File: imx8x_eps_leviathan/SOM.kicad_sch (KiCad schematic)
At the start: 3 parts, among them J10 BTH-070-02-L-D-A, J9 BTH-070-02-L-D-A (A to B)

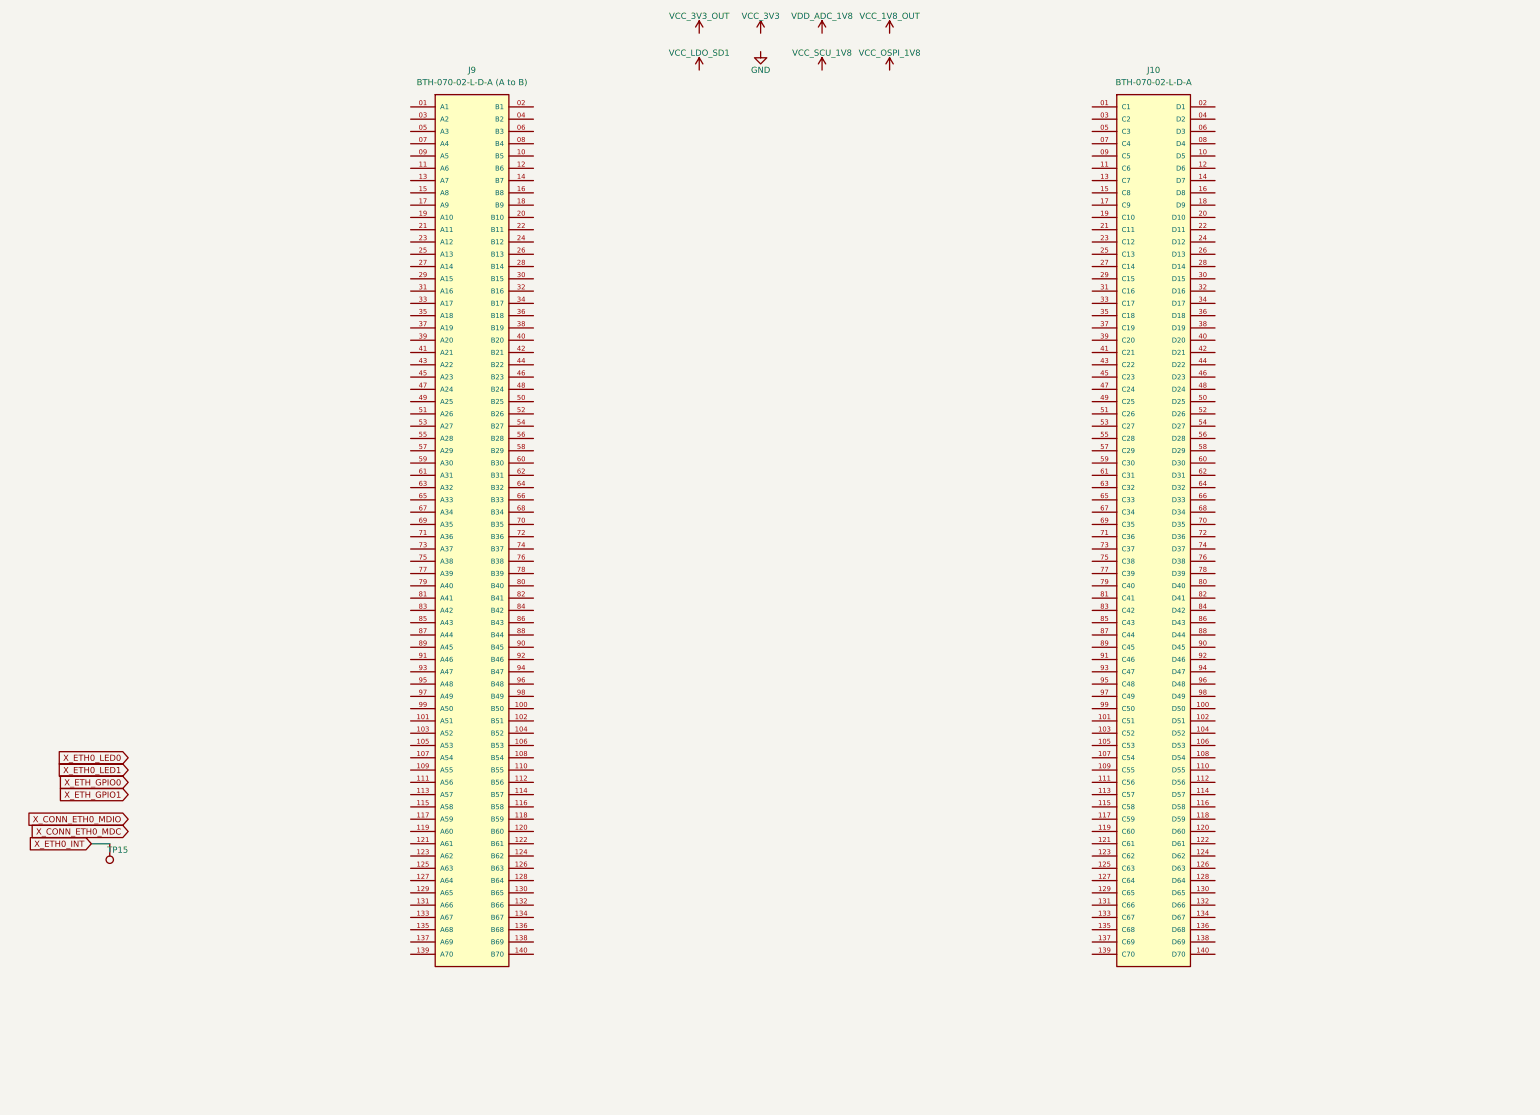
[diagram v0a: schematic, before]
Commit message: good stufff
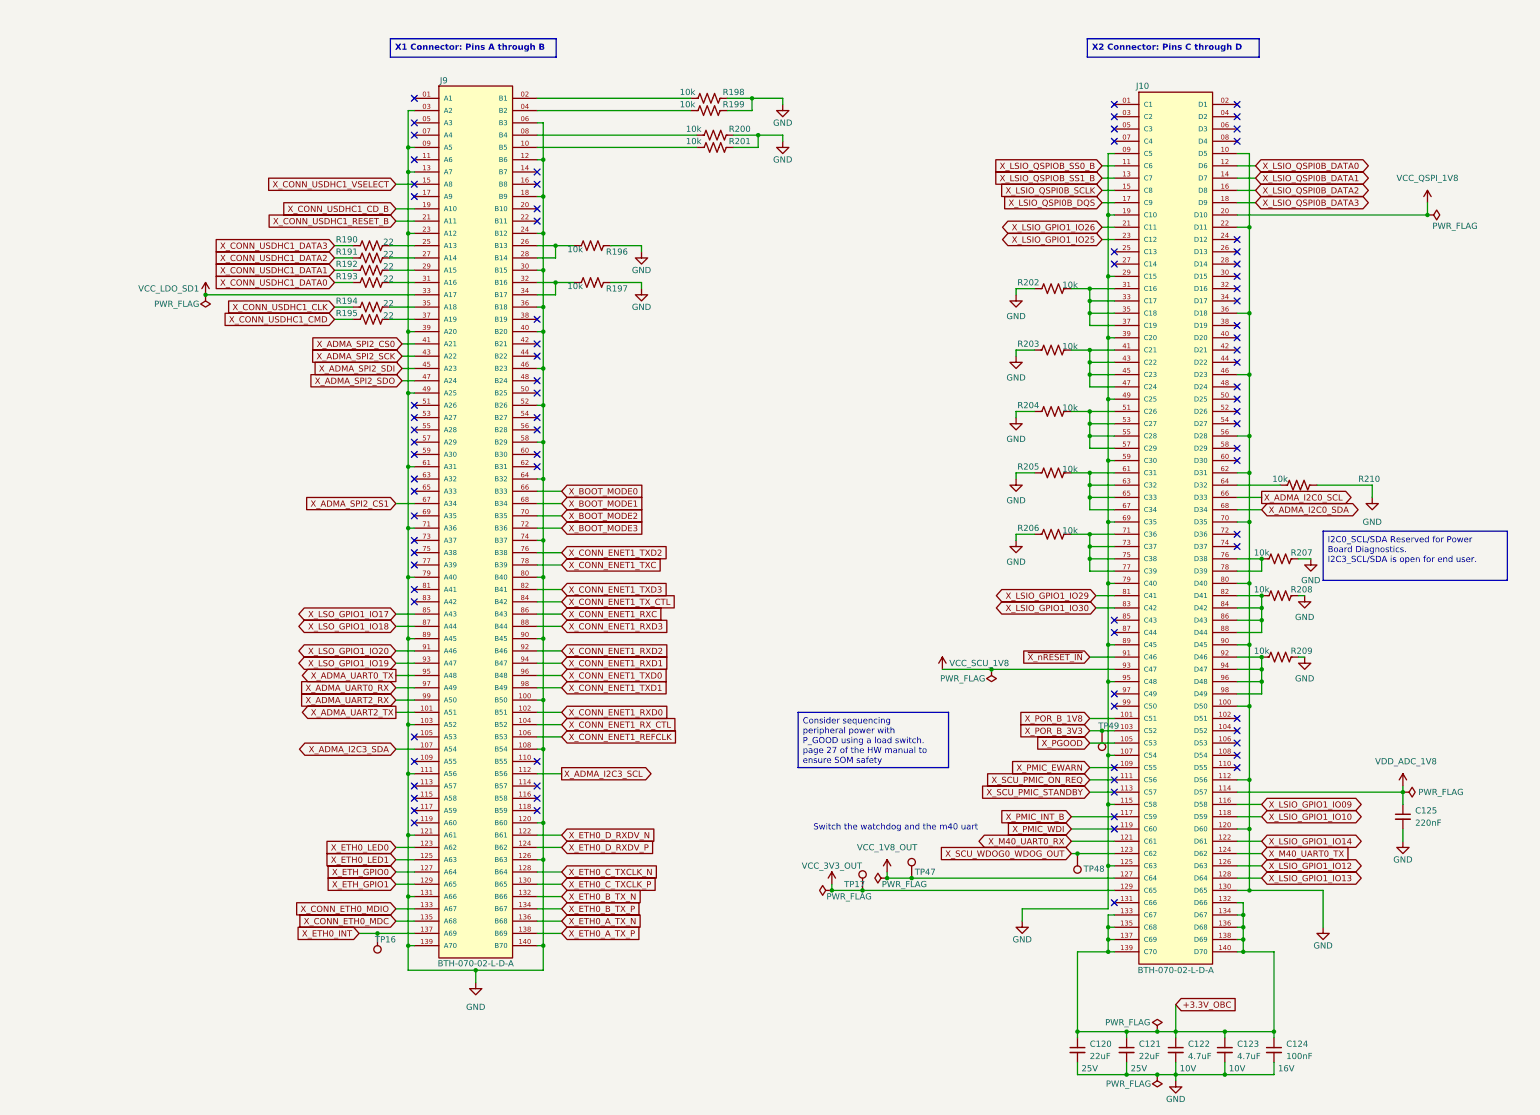
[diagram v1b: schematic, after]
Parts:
- removed TP15: TestPoint, TestPoint:TestPoint_THTPad_1.0x1.0mm_Drill0.5mm, symbol Connector:TestPoint
- added C120, C121: 22uF, Capacitor_SMD:C_0603_1608Metric, symbol Device:C_Small
- added C122, C123: 4.7uF, Capacitor_SMD:C_0603_1608Metric, symbol Device:C_Small
- added C124: 100nF, Capacitor_SMD:C_0603_1608Metric, symbol Device:C_Small
- added C125: 220nF, Capacitor_SMD:C_0603_1608Metric, symbol Device:C_Small
- added R190, R191, R192, R193, R194, R195: 22, Resistor_SMD:R_0402_1005Metric, symbol Device:R_US
- added R196, R197, R198, R199, R200, R201, R202, R203, R204, R205, R206, R207, R208, R209, R210: 10k, Resistor_SMD:R_0402_1005Metric, symbol Device:R_US
- added TP16, TP17, TP47, TP48, TP49: TestPoint, TestPoint:TestPoint_THTPad_1.0x1.0mm_Drill0.5mm, symbol Connector:TestPoint
- J9: value BTH-070-02-L-D-A (A to B) -> BTH-070-02-L-D-A
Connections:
- net GND: now also J10.09 (C5), J10.10 (D5), J10.100 (D50), J10.107 (C54), J10.112 (D56), J10.115 (C58), J10.120 (D60), J10.125 (C63), J10.130 (D65), J10.19 (C10), J10.22 (D11), J10.29 (C15), J10.36 (D18), J10.39 (C20), J10.46 (D23), J10.49 (C25), J10.56 (D28), J10.59 (C30), J10.62 (D31), J10.69 (C35), J10.70 (D35), J10.79 (C40), J10.80 (D40), J10.89 (C45), J10.90 (D45), J10.95 (C48), J9.03 (A2), J9.06 (B3), J9.09 (A5), J9.100 (B50), J9.103 (A52), J9.108 (B54), J9.111 (A56), J9.12 (B6), J9.120 (B60), J9.121 (A61), J9.126 (B63), J9.13 (A7), J9.131 (A66), J9.139 (A70), J9.140 (B70), J9.18 (B9), J9.23 (A12), J9.24 (B12), J9.30 (B15), J9.36 (B18), J9.39 (A20), J9.40 (B20), J9.46 (B23), J9.49 (A25), J9.52 (B26), J9.58 (B29), J9.61 (A31), J9.64 (B32), J9.71 (A36), J9.74 (B37), J9.79 (A40), J9.80 (B40), J9.89 (A45), J9.90 (B45), C120.2, C121.2, C122.2, C123.2, C124.2, C125.2, R196.1, R197.1, R198.1, R199.1, R200.1, R201.1, R202.1, R203.1, R204.1, R205.1, R206.1, R207.1, R208.1, R209.1, R210.1
- net VCC_1V8_OUT: now also J10.127 (C64), TP47.1
- net VCC_3V3_OUT: now also J10.129 (C65), TP17.1
- net VCC_LDO_SD1: now also J9.33 (A17)
- net VCC_SCU_1V8: now also J10.93 (C47)
- net VDD_ADC_1V8: now also J10.114 (D57), C125.1
- net X_CONN_ETH0_MDC: now also J9.135 (A68)
- net X_CONN_ETH0_MDIO: now also J9.133 (A67)
- net X_ETH0_INT: now also J9.137 (A69), TP16.1
- net X_ETH0_LED0: now also J9.123 (A62)
- net X_ETH0_LED1: now also J9.125 (A63)
- net X_ETH_GPIO0: now also J9.127 (A64)
- net X_ETH_GPIO1: now also J9.129 (A65)
- net X_POR_B_1V8: now reaches J10.101 (C51)
- net X_POR_B_3V3: now reaches J10.103 (C52)
- net X_POR_B_3V3: now also TP49.1
- net X_PGOOD: now reaches J10.105 (C53)
- net X_PMIC_EWARN: now reaches J10.109 (C55)
- net X_LSIO_QSPIOB_SS0_B: now reaches J10.11 (C6)
- net X_SCU_PMIC_ON_REQ: now reaches J10.111 (C56)
- net X_SCU_PMIC_STANDBY: now reaches J10.113 (C57)
- net X_LSIO_GPIO1_IO09: now reaches J10.116 (D58)
- net X_PMIC_INT_B: now reaches J10.117 (C59)
- net X_LSIO_GPIO1_IO10: now reaches J10.118 (D59)
- net X_PMIC_WDI: now reaches J10.119 (C60)
- net X_LSIO_QSPI0B_DATA0: now reaches J10.12 (D6)
- net X_M40_UART0_RX: now reaches J10.121 (C61)
- net X_LSIO_GPIO1_IO14: now reaches J10.122 (D61)
- net X_SCU_WDOG0_WDOG_OUT: now reaches J10.123 (C62)
- net X_SCU_WDOG0_WDOG_OUT: now also TP48.1
- net X_M40_UART0_TX: now reaches J10.124 (D62)
- net X_LSIO_GPIO1_IO12: now reaches J10.126 (D63)
- net X_LSIO_GPIO1_IO13: now reaches J10.128 (D64)
- net X_LSIO_QSPIOB_SS1_B: now reaches J10.13 (C7)
- net +3.3V_OBC: now reaches J10.132 (D66)
- net +3.3V_OBC: now also J10.133 (C67), J10.134 (D67), J10.135 (C68), J10.136 (D68), J10.137 (C69), J10.138 (D69), J10.139 (C70), J10.140 (D70), C120.1, C121.1, C122.1, C123.1, C124.1
- net X_LSIO_QSPI0B_DATA1: now reaches J10.14 (D7)
- net X_LSIO_QSPI0B_SCLK: now reaches J10.15 (C8)
- net X_LSIO_QSPI0B_DATA2: now reaches J10.16 (D8)
- net X_LSIO_QSPI0B_DQS: now reaches J10.17 (C9)
- net X_LSIO_QSPI0B_DATA3: now reaches J10.18 (D9)
- net VCC_QSPI_1V8: now reaches J10.20 (D10)
- net X_LSIO_GPIO1_IO26: now reaches J10.21 (C11)
- net X_LSIO_GPIO1_IO25: now reaches J10.23 (C12)
- net at J10.31 (C16): now also J10.33 (C17), J10.35 (C18), J10.37 (C19), R202.2
- net at J10.41 (C21): now also J10.43 (C22), J10.45 (C23), J10.47 (C24), R203.2
- net at J10.51 (C26): now also J10.53 (C27), J10.55 (C28), J10.57 (C29), R204.2
- net at J10.61 (C31): now also J10.63 (C32), J10.65 (C33), J10.67 (C34), R205.2
- net at J10.64 (D32): now also R210.2
- net X_ADMA_I2C0_SCL: now reaches J10.66 (D33)
- net X_ADMA_I2C0_SDA: now reaches J10.68 (D34)
- net at J10.71 (C36): now also J10.73 (C37), J10.75 (C38), J10.77 (C39), R206.2
- net at J10.76 (D38): now also J10.78 (D39), R207.2
- net X_LSIO_GPIO1_IO29: now reaches J10.81 (C41)
- net at J10.82 (D41): now also J10.84 (D42), J10.86 (D43), J10.88 (D44), R208.2
- net X_LSIO_GPIO1_IO30: now reaches J10.83 (C42)
- net ~{X_nRESET_IN}: now reaches J10.91 (C46)
- net at J10.92 (D46): now also J10.94 (D47), J10.96 (D48), J10.98 (D49), R209.2
- net at J9.02 (B1): now also R198.2
- net at J9.04 (B2): now also R199.2
- net at J9.08 (B4): now also R200.2
- net at J9.10 (B5): now also R201.2
- net X_ADMA_UART2_TX: now reaches J9.101 (A51)
- net X_CONN_ENET1_RXD0: now reaches J9.102 (B51)
- net X_CONN_ENET1_RX_CTL: now reaches J9.104 (B52)
- net X_CONN_ENET1_REFCLK: now reaches J9.106 (B53)
- net X_ADMA_I2C3_SDA: now reaches J9.107 (A54)
- net X_ADMA_I2C3_SCL: now reaches J9.112 (B56)
- net X_ETH0_D_RXDV_N: now reaches J9.122 (B61)
- net X_ETH0_D_RXDV_P: now reaches J9.124 (B62)
- net X_ETH0_C_TXCLK_N: now reaches J9.128 (B64)
- net X_ETH0_C_TXCLK_P: now reaches J9.130 (B65)
- net X_ETH0_B_TX_N: now reaches J9.132 (B66)
- net X_ETH0_B_TX_P: now reaches J9.134 (B67)
- net X_ETH0_A_TX_N: now reaches J9.136 (B68)
- net X_ETH0_A_TX_P: now reaches J9.138 (B69)
- net X_CONN_USDHC1_VSELECT: now reaches J9.15 (A8)
- net X_CONN_USDHC1_CD_B: now reaches J9.19 (A10)
- net X_CONN_USDHC1_RESET_B: now reaches J9.21 (A11)
- net at J9.25 (A13): now also R190.2
- net at J9.26 (B13): now also J9.28 (B14), R196.2
- net at J9.27 (A14): now also R191.2
- net at J9.29 (A15): now also R192.2
- net at J9.31 (A16): now also R193.2
- net at J9.32 (B16): now also J9.34 (B17), R197.2
- net at J9.35 (A18): now also R194.2
- net at J9.37 (A19): now also R195.2
- net X_ADMA_SPI2_CS0: now reaches J9.41 (A21)
- net X_ADMA_SPI2_SCK: now reaches J9.43 (A22)
- net X_ADMA_SPI2_SDI: now reaches J9.45 (A23)
- net X_ADMA_SPI2_SDO: now reaches J9.47 (A24)
- net X_BOOT_MODE0: now reaches J9.66 (B33)
- net X_ADMA_SPI2_CS1: now reaches J9.67 (A34)
- net X_BOOT_MODE1: now reaches J9.68 (B34)
- net X_BOOT_MODE2: now reaches J9.70 (B35)
- net X_BOOT_MODE3: now reaches J9.72 (B36)
- net X_CONN_ENET1_TXD2: now reaches J9.76 (B38)
- net X_CONN_ENET1_TXC: now reaches J9.78 (B39)
- net X_CONN_ENET1_TXD3: now reaches J9.82 (B41)
- net X_CONN_ENET1_TX_CTL: now reaches J9.84 (B42)
- net X_LSO_GPIO1_IO17: now reaches J9.85 (A43)
- net X_CONN_ENET1_RXC: now reaches J9.86 (B43)
- net X_LSO_GPIO1_IO18: now reaches J9.87 (A44)
- net X_CONN_ENET1_RXD3: now reaches J9.88 (B44)
- net X_LSO_GPIO1_IO20: now reaches J9.91 (A46)
- net X_CONN_ENET1_RXD2: now reaches J9.92 (B46)
- net X_LSO_GPIO1_IO19: now reaches J9.93 (A47)
- net X_CONN_ENET1_RXD1: now reaches J9.94 (B47)
- net X_ADMA_UART0_TX: now reaches J9.95 (A48)
- net X_CONN_ENET1_TXD0: now reaches J9.96 (B48)
- net X_ADMA_UART0_RX: now reaches J9.97 (A49)
- net X_CONN_ENET1_TXD1: now reaches J9.98 (B49)
- net X_ADMA_UART2_RX: now reaches J9.99 (A50)
- new net X_CONN_USDHC1_CLK: R194.1
- new net X_CONN_USDHC1_CMD: R195.1
- new net X_CONN_USDHC1_DATA0: R193.1
- new net X_CONN_USDHC1_DATA1: R192.1
- new net X_CONN_USDHC1_DATA2: R191.1
- new net X_CONN_USDHC1_DATA3: R190.1
- no-connect marks 0 -> 85
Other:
- note added: "Switch the watchdog and the m40 uart"

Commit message: bruh
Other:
- title: (none) -> Leviathan 1-A
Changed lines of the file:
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@@
 	(paper "A3")
 	(title_block
+		(title "Leviathan 1-A")
+		(date "2025-10-22")
+		(rev "1-A")
 		(company "Bronco Space Lab")
 		(comment 1 "By John Pollak & Luca Lanzillotta")

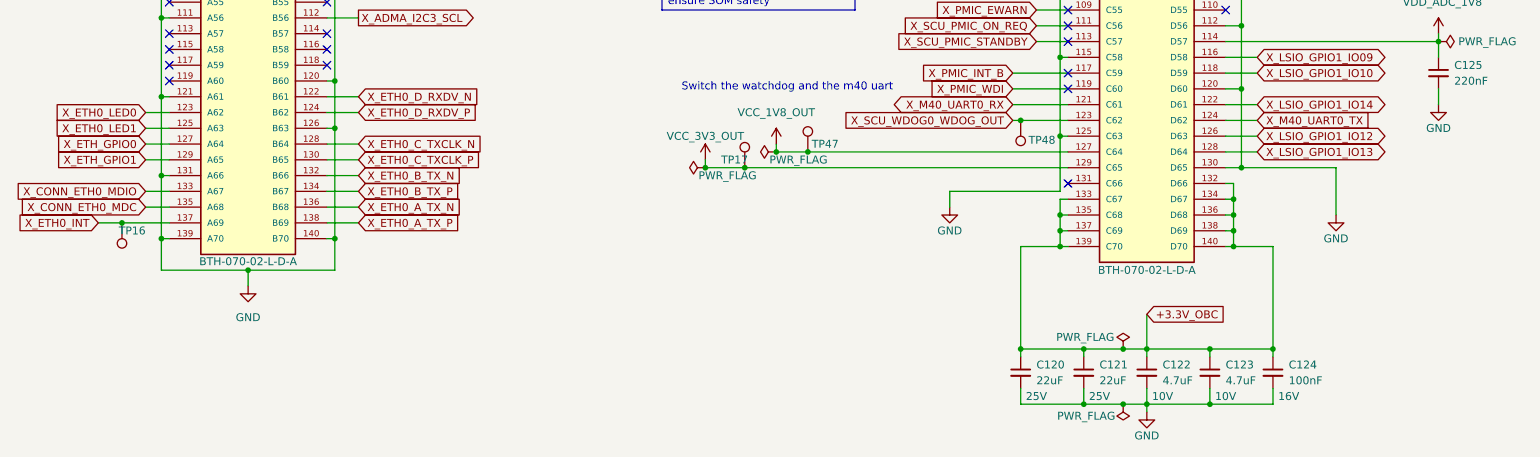
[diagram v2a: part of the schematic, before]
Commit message: Updated Schematic and SOM
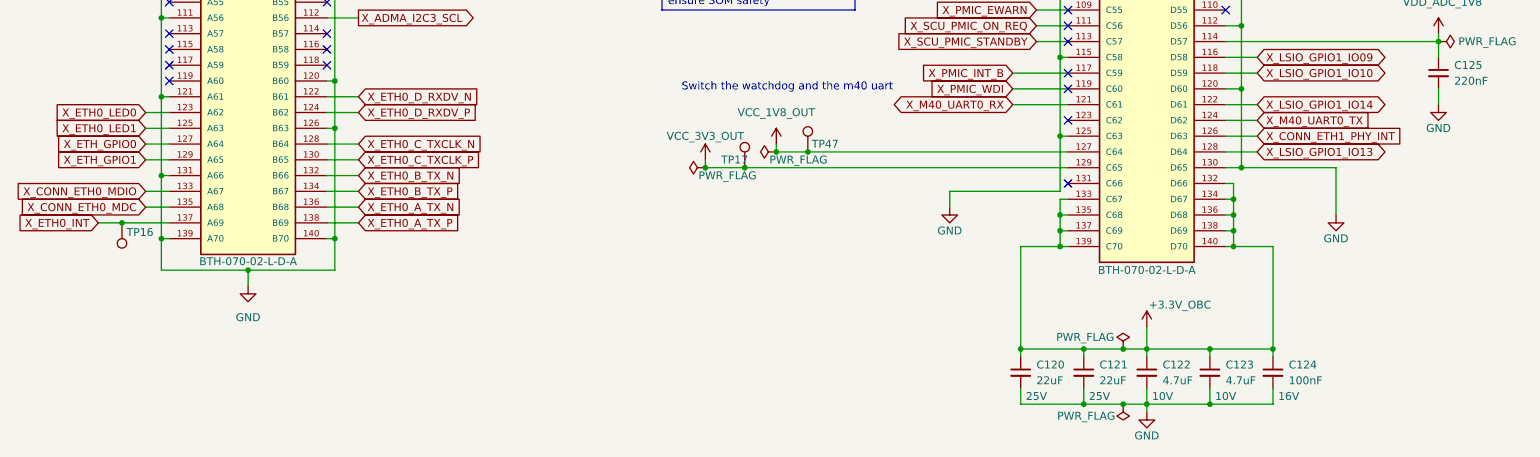
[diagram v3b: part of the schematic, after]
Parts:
- removed TP48: TestPoint, TestPoint:TestPoint_THTPad_1.0x1.0mm_Drill0.5mm, symbol Connector:TestPoint
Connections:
- net X_LSIO_GPIO1_IO12 renamed X_CONN_ETH1_PHY_INT
- net X_SCU_WDOG0_WDOG_OUT: no longer names the net of J10.123 (C62)
- no-connect marks 85 -> 86
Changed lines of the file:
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@@
 	)
 	(junction
-		(at 258.572 195.072)
-		(diameter 0)
-		(color 0 0 0 0)
-	)
-	(junction
 		(at 292.862 212.852)
 		(diameter 0)
@@
 	)
 	(no_connect
+		(at 266.192 195.072)
+	)
+	(no_connect
 		(at 291.592 167.132)
 	)
@@
 	(wire
 		(pts
-			(xy 278.892 226.314) (xy 278.892 231.902)
+			(xy 278.892 228.346) (xy 278.892 231.902)
 		)
 		(stroke
@@
 	(wire
 		(pts
-			(xy 257.302 195.072) (xy 258.572 195.072)
-		)
-		(stroke
-			(width 0)
-			(type default)
-		)
-	)
-	(wire
-		(pts
 			(xy 120.142 115.062) (xy 120.142 127.762)
 		)
@@
 	(wire
 		(pts
-			(xy 258.572 195.072) (xy 266.192 195.072)
-		)
-		(stroke
-			(width 0)
-			(type default)
-		)
-	)
-	(wire
-		(pts
 			(xy 261.112 182.372) (xy 266.192 182.372)
 		)
@@
 		)
 	)
-	(global_label "X_LSIO_GPIO1_IO12"
-		(shape bidirectional)
-		(at 296.672 197.612 0)
-		(fields_autoplaced yes)
-		(effects
-			(font
-				(size 1.27 1.27)
-			)
-			(justify left)
-		)
-		(property "Intersheetrefs" "${INTERSHEET_REFS}"
-			(at 319.0928 197.612 0)
-			(effects
-				(font
-					(size 1.27 1.27)
-				)
-				(justify left)
-				(hide yes)
-			)
-		)
-	)
 	(global_label "X_CONN_ENET1_RX_CTL"
 		(shape input)
@@
 		)
 	)
-	(global_label "+3.3V_OBC"
+	(global_label "X_CONN_ETH1_PHY_INT"
 		(shape input)
-		(at 278.892 226.314 0)
+		(at 296.672 197.612 0)
 		(fields_autoplaced yes)
 		(effects
@@
 		)
 		(property "Intersheetrefs" "${INTERSHEET_REFS}"
-			(at 292.4001 226.314 0)
+			(at 321.2472 197.612 0)
 			(effects
 				(font
@@
 		)
 	)
-	(global_label "X_SCU_WDOG0_WDOG_OUT"
-		(shape input)
-		(at 257.302 195.072 180)
-		(fields_autoplaced yes)
-		(effects
-			(font
-				(size 1.27 1.27)
-			)
-			(justify right)
-		)
-		(property "Intersheetrefs" "${INTERSHEET_REFS}"
-			(at 229.945 195.072 0)
-			(effects
-				(font
-					(size 1.27 1.27)
-				)
-				(justify right)
-				(hide yes)
-			)
-		)
-	)
 	(global_label "X_BOOT_MODE1"
 		(shape input)
@@
 	)
 	(symbol
-		(lib_id "Connector:TestPoint")
-		(at 258.572 195.072 180)
-		(unit 1)
-		(exclude_from_sim no)
-		(in_bom yes)
-		(on_board yes)
-		(dnp no)
-		(property "Reference" "TP48"
-			(at 259.842 198.247 0)
-			(effects
-				(font
-					(size 1.27 1.27)
-				)
-				(justify right)
-			)
-		)
-		(property "Value" "TestPoint"
-			(at 261.112 199.6439 0)
-			(effects
-				(font
-					(size 1.27 1.27)
-				)
-				(justify right)
-				(hide yes)
-			)
-		)
-		(property "Footprint" "TestPoint:TestPoint_THTPad_1.0x1.0mm_Drill0.5mm"
-			(at 253.492 195.072 0)
-			(effects
-				(font
-					(size 1.27 1.27)
-				)
-				(hide yes)
-			)
-		)
-		(property "Datasheet" "~"
-			(at 253.492 195.072 0)
-			(effects
-				(font
-					(size 1.27 1.27)
-				)
-				(hide yes)
-			)
-		)
-		(property "Description" "test point"
-			(at 258.572 195.072 0)
-			(effects
-				(font
-					(size 1.27 1.27)
-				)
-				(hide yes)
-			)
-		)
-		(property "LCSC" ""
-			(at 258.572 195.072 0)
-			(effects
-				(font
-					(size 1.27 1.27)
-				)
-			)
-		)
-		(property "Voltage" ""
-			(at 258.572 195.072 0)
-			(effects
-				(font
-					(size 1.27 1.27)
-				)
-			)
-		)
-		(pin "1"
-		)
-		(instances
-			(project "imx8x_eps_leviathan"
-				(path "/bd3af9f3-19df-4a2f-8b54-98c48cea082e/1b5b2e76-614d-4307-9232-e06f7c77302d/d76dd75e-585c-4f61-92c5-bda4099b5574"
-					(reference "TP48")
-					(unit 1)
-				)
-			)
-		)
-	)
-	(symbol
 		(lib_id "Device:R_US")
 		(at 112.522 74.422 90)
@@
 		(dnp no)
 		(property "Reference" "TP16"
-			(at 117.602 212.852 0)
+			(at 118.872 213.106 0)
 			(effects
 				(font
@@
 					(unit 1)
 				)
+			)
+		)
+	)
+	(symbol
+		(lib_id "power:+3.3V")
+		(at 278.892 228.346 0)
+		(unit 1)
+		(exclude_from_sim no)
+		(in_bom yes)
+		(on_board yes)
+		(dnp no)
+		(property "Reference" "#PWR0170"
+			(at 278.892 232.156 0)
+			(effects
+				(font
+					(size 1.27 1.27)
+				)
+				(hide yes)
+			)
+		)
+		(property "Value" "+3.3V_OBC"
+			(at 284.226 224.79 0)
+			(effects
+				(font
+					(size 1.27 1.27)
+				)
+			)
+		)
+		(property "Footprint" ""
+			(at 278.892 228.346 0)
+			(effects
+				(font
+					(size 1.27 1.27)
+				)
+				(hide yes)
+			)
+		)
+		(property "Datasheet" ""
+			(at 278.892 228.346 0)
+			(effects
+				(font
+					(size 1.27 1.27)
+				)
+				(hide yes)
+			)
+		)
+		(property "Description" "Power symbol creates a global label with name \"+3.3V\""
+			(at 278.892 228.346 0)
+			(effects
+				(font
+					(size 1.27 1.27)
+				)
+				(hide yes)
+			)
+		)
+		(pin "1"
+		)
+		(instances
+			(project "imx8x_eps_leviathan"
+				(path "/bd3af9f3-19df-4a2f-8b54-98c48cea082e/1b5b2e76-614d-4307-9232-e06f7c77302d/d76dd75e-585c-4f61-92c5-bda4099b5574"
+					(reference "#PWR0170")
+					(unit 1)
+				)
